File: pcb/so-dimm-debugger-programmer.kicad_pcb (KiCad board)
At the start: 2 copper layers, 131.2 x 48.9 mm, 49 parts, among them J1 1612618-4, J10 Conn_01x08_Male, J11 Conn_01x08_Male, J12 UART, J13 Conn_01x04_Pin, J2 V0_SPI, J3 V1_SPI, J4 I2C_0, J5 I2C_1, J6 USB4105-GF-A, J7 USB4105-GF-A, J8 Conn_02x16_Odd_Even, Q1 UMH3N, SW1 SW_Push, SW2 SW_Push, U1 AP2112K-3.3, U2 USBLC6-2P6, U3 USBLC6-2P6, U4 CP2102N-Axx-xQFN28

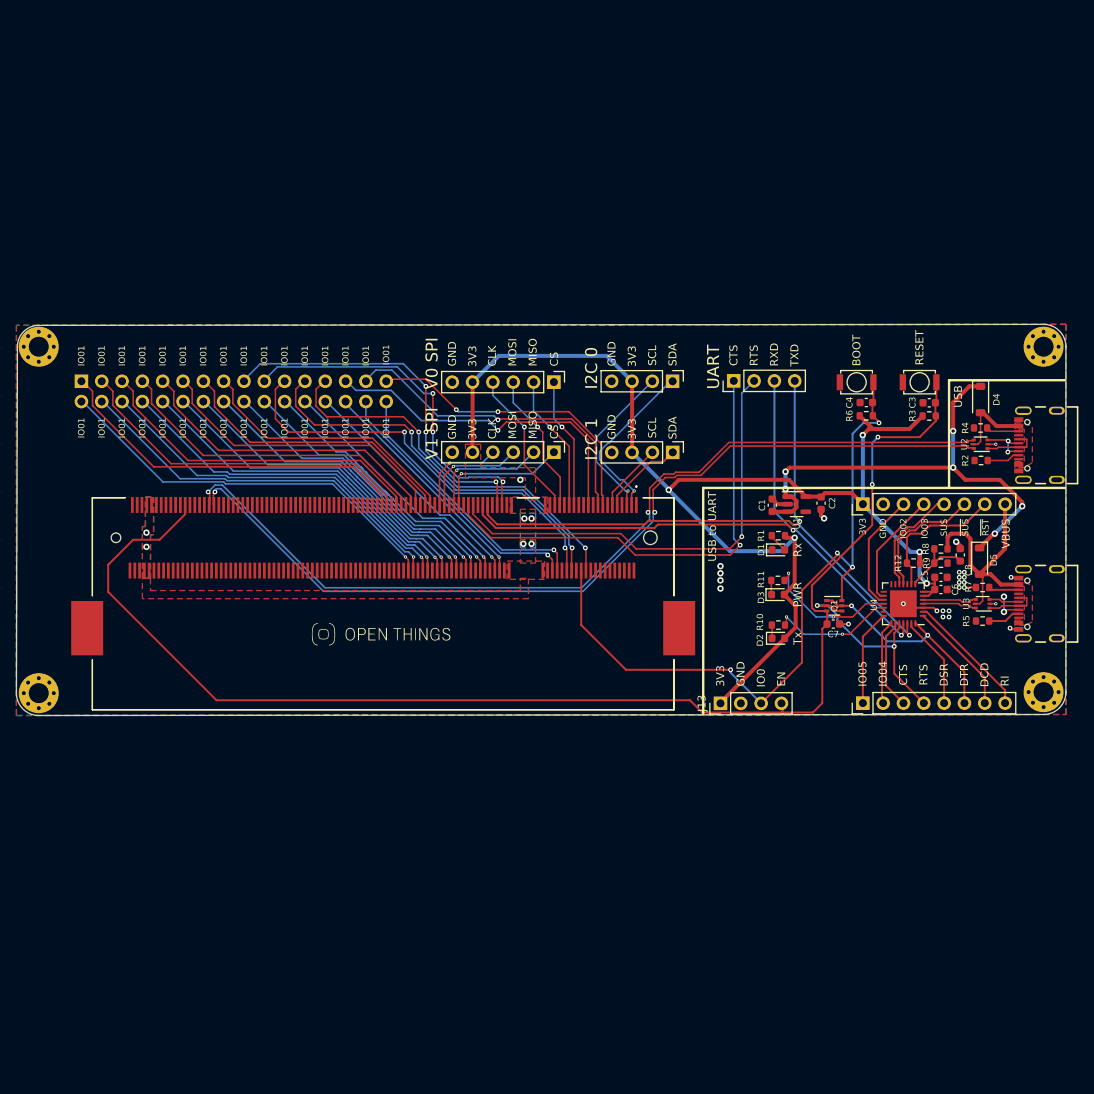
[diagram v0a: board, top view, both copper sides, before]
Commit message: Finished up board layout
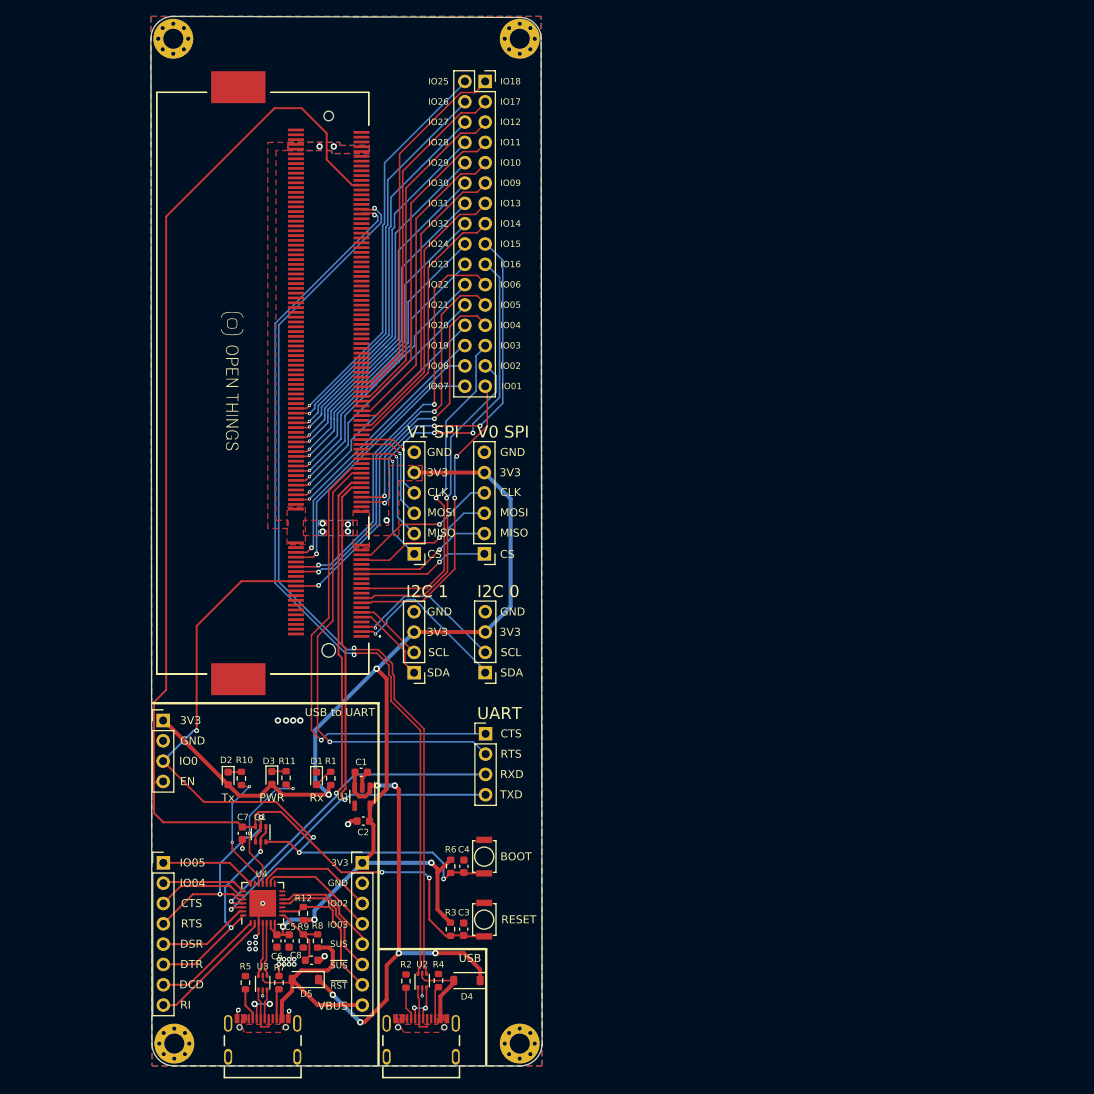
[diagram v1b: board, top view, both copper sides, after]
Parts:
- moved H1 117.2 mm to (96.7, 166.0), turned to -90 degrees
- moved J7 114.3 mm to (107.8, 167.6), turned to 0 degrees
- moved J6 110.3 mm to (127.6, 167.6), turned to 0 degrees
- moved H3 109.0 mm to (139.9, 166.0), turned to -90 degrees
- moved R5 102.6 mm to (105.6, 158.4), turned to -90 degrees
- moved U3 101.7 mm to (107.8, 158.4), turned to 90 degrees
- moved R7 100.9 mm to (109.8, 158.4), turned to -90 degrees
- moved D5 99.2 mm to (113.1, 158.0), turned to 180 degrees
- moved R2 97.0 mm to (125.7, 158.2), turned to -90 degrees
- moved D4 96.9 mm to (133.3, 158.1), turned to 180 degrees
- moved U2 96.8 mm to (127.7, 158.1), turned to 90 degrees
- moved R4 96.8 mm to (129.7, 158.1), turned to -90 degrees
- moved C8 95.6 mm to (113.9, 155.6), turned to 0 degrees
- moved C6 93.9 mm to (109.5, 153.1), turned to -90 degrees
- moved C5 93.3 mm to (111.1, 153.1), turned to -90 degrees
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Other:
- board size 131.2 x 48.9 mm -> 48.9 x 131.2 mm
- board text added: "IO06"
- board text added: "IO07"
- board text added: "IO08"
- board text added: "IO09"
- board text added: "IO10"
- board text added: "IO11"
- board text added: "IO12"
- board text added: "IO13"
- board text added: "IO14"
- board text added: "IO15"
- board text added: "IO16"
- board text added: "IO17"
- board text added: "IO18"
- board text added: "IO19"
- board text added: "IO20"
- board text added: "IO21"
- board text added: "IO22"
- board text added: "IO23"
- board text added: "IO24"
- board text added: "IO25"
- board text added: "IO26"
- board text added: "IO27"
- board text added: "IO28"
- board text added: "IO29"
- board text added: "IO30"
- board text added: "IO31"
- board text added: "IO32"
